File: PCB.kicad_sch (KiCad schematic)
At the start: 52 parts, among them J1 USB_C_Receptacle_USB2.0_16P, J10 Conn_01x06_Socket, J11 Conn_01x02_Pin, J13 Conn_01x05_Pin, J2 Conn_01x06_Socket, J3 Conn_01x04_Pin, J4 Conn_01x05_Pin, J5 Conn_01x02_Pin, J6 Conn_01x02_Pin, J7 Conn_01x02_Pin, J8 Conn_01x04_Pin, J9 Conn_01x05_Pin, SW1 SW_Push, SW2 SW_Push, U1 TMC2209_SILENTSTEPSTICK, U2 USBLC6-2SC6, U4 AMS1117-3.3 (UMW), U5 TMC2209_SILENTSTEPSTICK, U6 ESP32-S3-WROOM-1

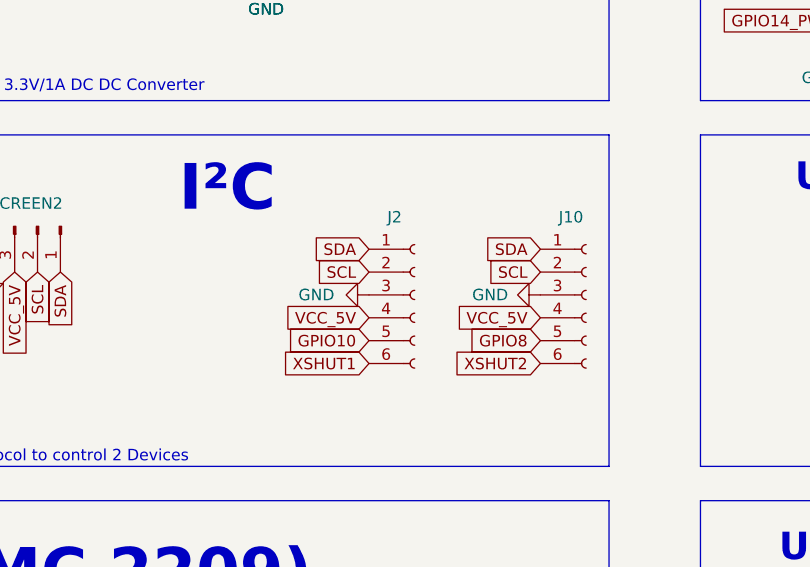
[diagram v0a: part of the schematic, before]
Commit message: V3 Corrigée (ToF)
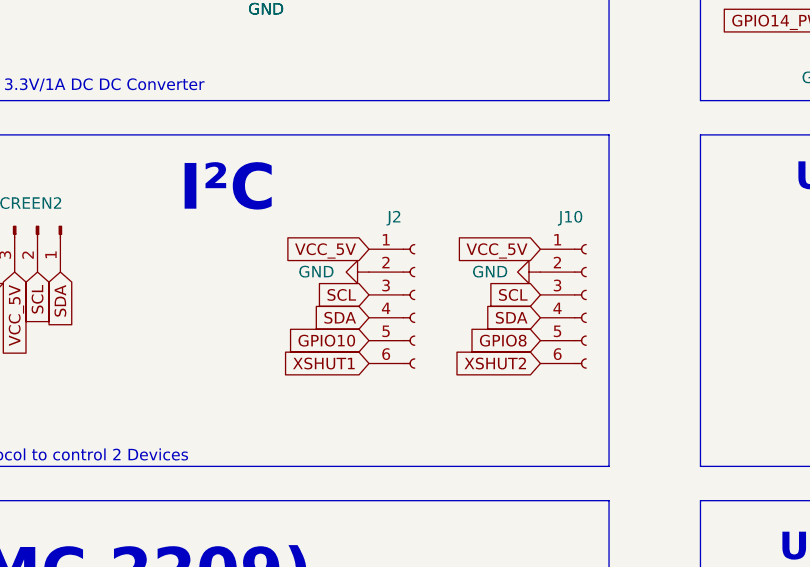
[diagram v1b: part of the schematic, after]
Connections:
- net GND: now also J10.2 (Pin_2), J2.2 (Pin_2); no longer J10.3 (Pin_3), J2.3 (Pin_3)
- net SCL: now also J10.3 (Pin_3), J2.3 (Pin_3); no longer J10.2 (Pin_2), J2.2 (Pin_2)
- net SDA: now also J10.4 (Pin_4), J2.4 (Pin_4); no longer J10.1 (Pin_1), J2.1 (Pin_1)
- net VCC_5V: now also J10.1 (Pin_1), J2.1 (Pin_1); no longer J10.4 (Pin_4), J2.4 (Pin_4)
